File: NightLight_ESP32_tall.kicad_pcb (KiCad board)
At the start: 2 copper layers, 30 x 120 mm, 27 parts, among them J1 USB_C_Receptacle_USB2.0, J2 BUTTON, Q1 MMBT2222, Q2 MMBT2222, SW1 TL3342, SW2 TL3342, U1 ESP32-WROOM-32D, U2 AP2112K-3.3, U3 CH340C

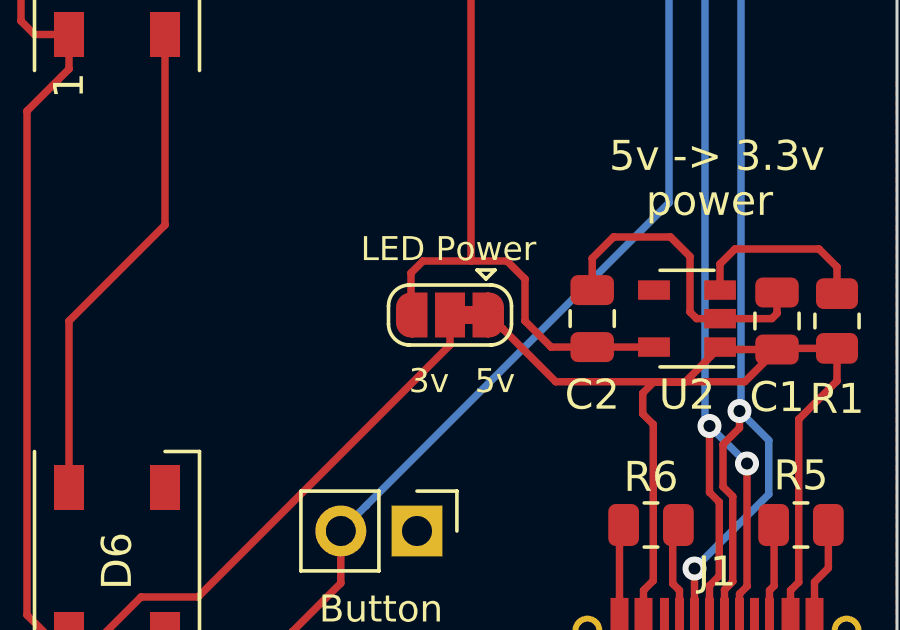
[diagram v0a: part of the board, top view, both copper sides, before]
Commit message: Updated to v6
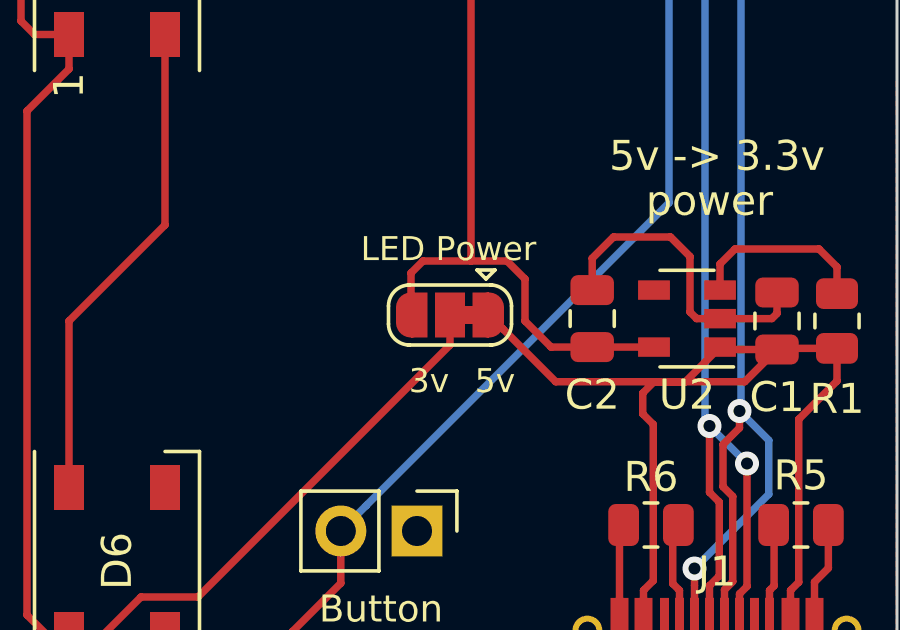
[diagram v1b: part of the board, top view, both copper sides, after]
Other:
- net class Default removed
